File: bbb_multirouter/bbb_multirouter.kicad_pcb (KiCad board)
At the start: 2 copper layers, 54.6 x 86.4 mm, 17 parts, among them CON1 CORTEX-DEBUGGER, J1 Conn_01x06, J2 Conn_01x02, J3 USB_C_Receptacle, J4 Conn_01x06, J5 Conn_01x10, P8 BeagleBone_Black_Header, P9 BeagleBone_Black_Header, SW1 SW_Push, SW2 SW_Push, SW3 SW_Push, U1 TRADFRI, U2 usbwifi

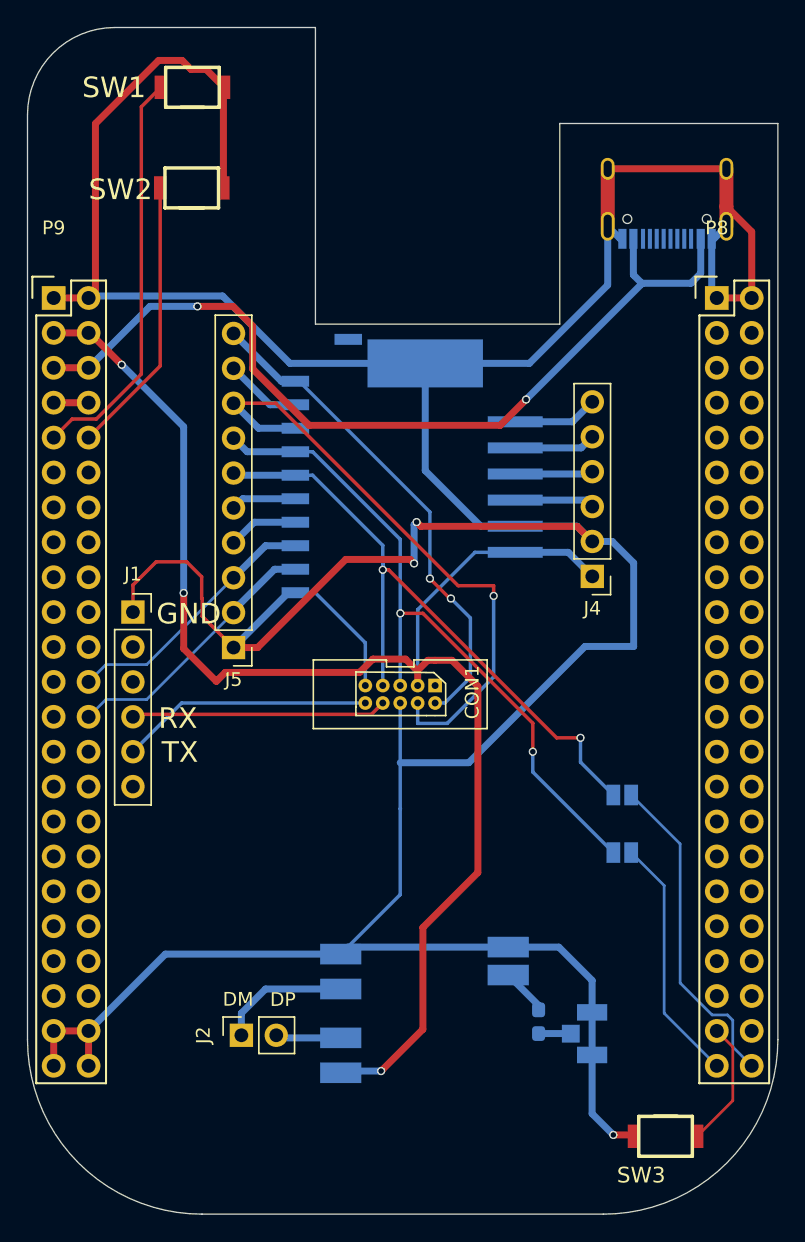
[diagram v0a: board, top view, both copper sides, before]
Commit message: usb wifi
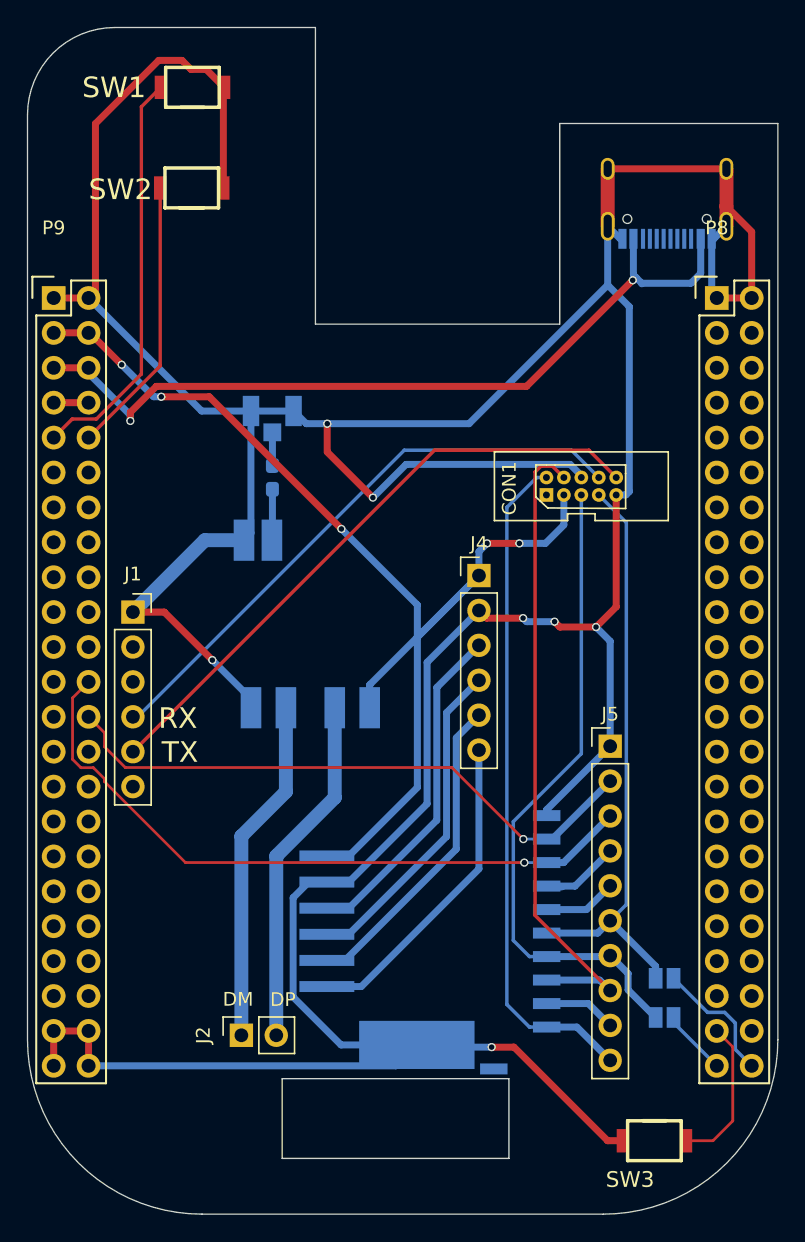
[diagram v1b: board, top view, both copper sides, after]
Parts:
- moved JP3 49.9 mm to (132.3, 71.4), turned to 180 degrees
- moved C1 44.1 mm to (132.3, 75.4), turned to 270 degrees
- moved U1 38.1 mm to (143.2, 111.0), turned to 270 degrees
- moved J5 28.3 mm to (156.9, 95.0), turned to 0 degrees
- moved U2 28.3 mm to (140.9, 92.2), turned to 90 degrees
- moved CON1 20.1 mm to (154.8, 76.1), turned to 90 degrees
- moved JP2 13.7 mm to (160.8, 111.9)
- moved JP1 12.4 mm to (160.8, 114.7)
- moved J4 8.25 mm to (147.3, 82.6), turned to 0 degrees
- moved SW3 0.87 mm to (160.1, 123.7)
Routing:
- net UART1_TXD: track 19.2 -> 49.9 mm, vias 0 -> 1
- net UART0_TX: track 18.4 -> 45.1 mm
- net UART0_RX: track 18.6 -> 43.0 mm
- net UART1_RXD: track 19.6 -> 44.0 mm, vias 0 -> 1
- net +3V3: track 108.7 -> 86.8 mm, vias 3 -> 5
- net USB_DP: track 4.77 -> 25.9 mm
- net /Sheet5FB19A08/PB13: track 5.80 -> 24.7 mm
- net /Sheet5FB19A08/PB12: track 5.68 -> 24.0 mm
- net /Sheet5FB19A08/I2C_SCL: track 5.95 -> 23.2 mm
- net /Sheet5FB19A08/I2C_SDA: track 6.21 -> 23.3 mm
- net USB_DM: track 9.57 -> 25.2 mm
- net LCD_DATA1: track 24.0 -> 9.45 mm
- net LCD_DATA0: track 18.1 -> 4.82 mm
- net RESETn: track 36.3 -> 49.2 mm, vias 2 -> 0
- net GND: track 311.8 -> 322.5 mm, vias 3 -> 7
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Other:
- outline, holes or cut-outs redrawn
- board text removed: "GND"
